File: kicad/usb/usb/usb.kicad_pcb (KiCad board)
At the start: 2 copper layers, 29.4 x 26 mm, 19 parts, among them J1 USB_C_Receptacle_USB2.0_14P, J2 PH1.25mm 2P, J3 Conn_01x07_Pin, Q1 BSS84, SW1 PWR, U1 S-T111B33MC-OGSTFU, U2 MCP73831-2-OT

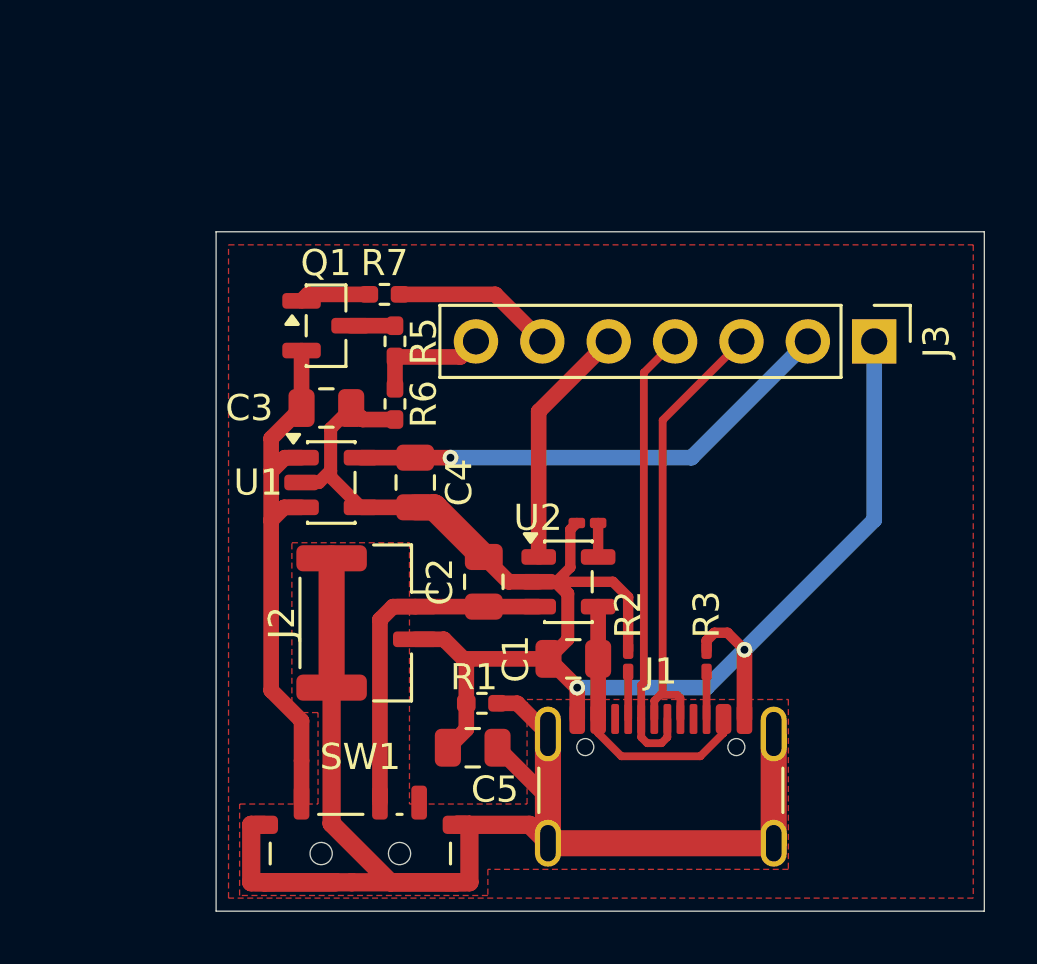
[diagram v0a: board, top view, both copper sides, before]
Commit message: Various kicad edits
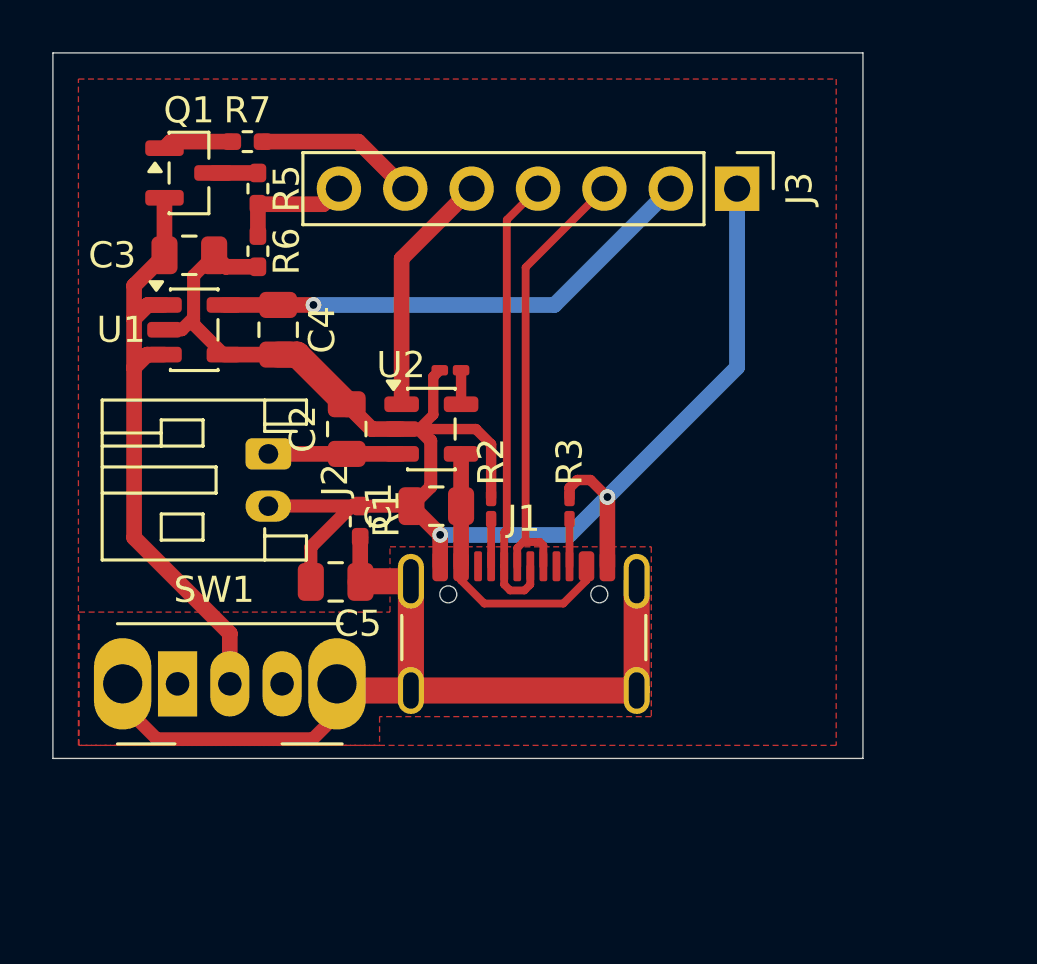
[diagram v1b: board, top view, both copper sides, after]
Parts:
- J2: value PH1.25mm 2P -> PH2.0mm 2P; footprint Connector_JST:JST_GH_SM02B-GHS-TB_1x02-1MP_P1.25mm_Horizontal -> Connector_JST:JST_PH_S2B-PH-K_1x02_P2.00mm_Horizontal
- SW1: footprint Button_Switch_SMD:SW_SPDT_Shouhan_MSK12C02 -> Button_Switch_THT:SW_Slide_SPDT_Angled_CK_OS102011MA1Q
- moved SW1 9.55 mm to (85.5, 112.3)
- moved R1 8.37 mm to (92.5, 106.1), turned to 90 degrees
- moved C5 8.23 mm to (91.6, 108.4)
- moved C1 7.85 mm to (95.4, 105.5)
- moved C2 7.85 mm to (92.0, 102.5)
- moved C3 7.85 mm to (86.0, 95.9)
- moved C4 7.85 mm to (89.4, 98.8)
- moved J3 7.85 mm to (106.9, 93.3)
- moved R4 7.85 mm to (96.0, 100.3)
- moved R5 7.85 mm to (88.6, 93.3)
- moved R6 7.85 mm to (88.6, 95.7)
- moved U1 7.85 mm to (86.2, 98.8)
- moved U2 7.85 mm to (95.2, 102.5)
- moved J1 7.85 mm to (98.8, 111.5)
- moved Q1 7.85 mm to (86.0, 92.8)
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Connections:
- SW1 pad 1: VSENSE -> unconnected-(SW1-A-Pad1)
- SW1 pad 2: VBAT -> VSENSE
- SW1 pad 3: unconnected-(SW1-C-Pad3) -> VBAT
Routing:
- net SHIELD: track 58.3 -> 34.7 mm
- net VBAT: track 13.3 -> 5.10 mm
- net VSENSE: track 21.0 -> 23.4 mm
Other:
- board size 29.4 x 26 mm -> 31 x 27 mm
